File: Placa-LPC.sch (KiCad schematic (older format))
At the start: 17 parts, among them K1 CONN_3, P6 CONN_4X2, P7 CONN_8, P8 CONN_6, X1 12MHz

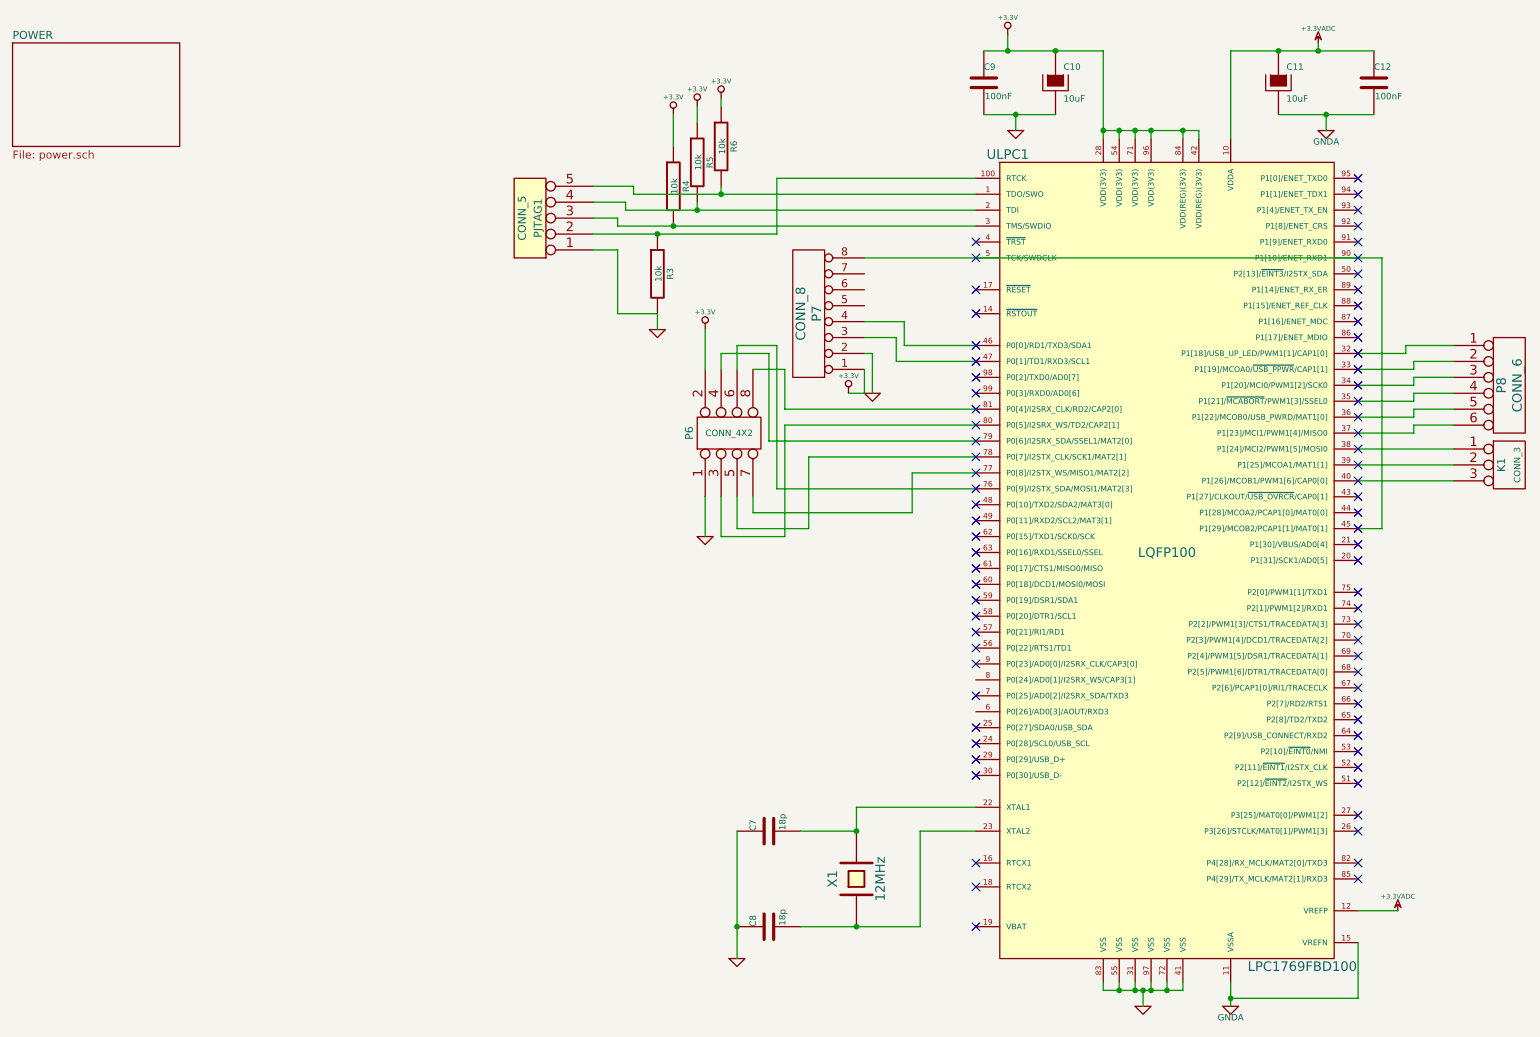
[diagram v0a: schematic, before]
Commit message: Actualizado desde mi pc
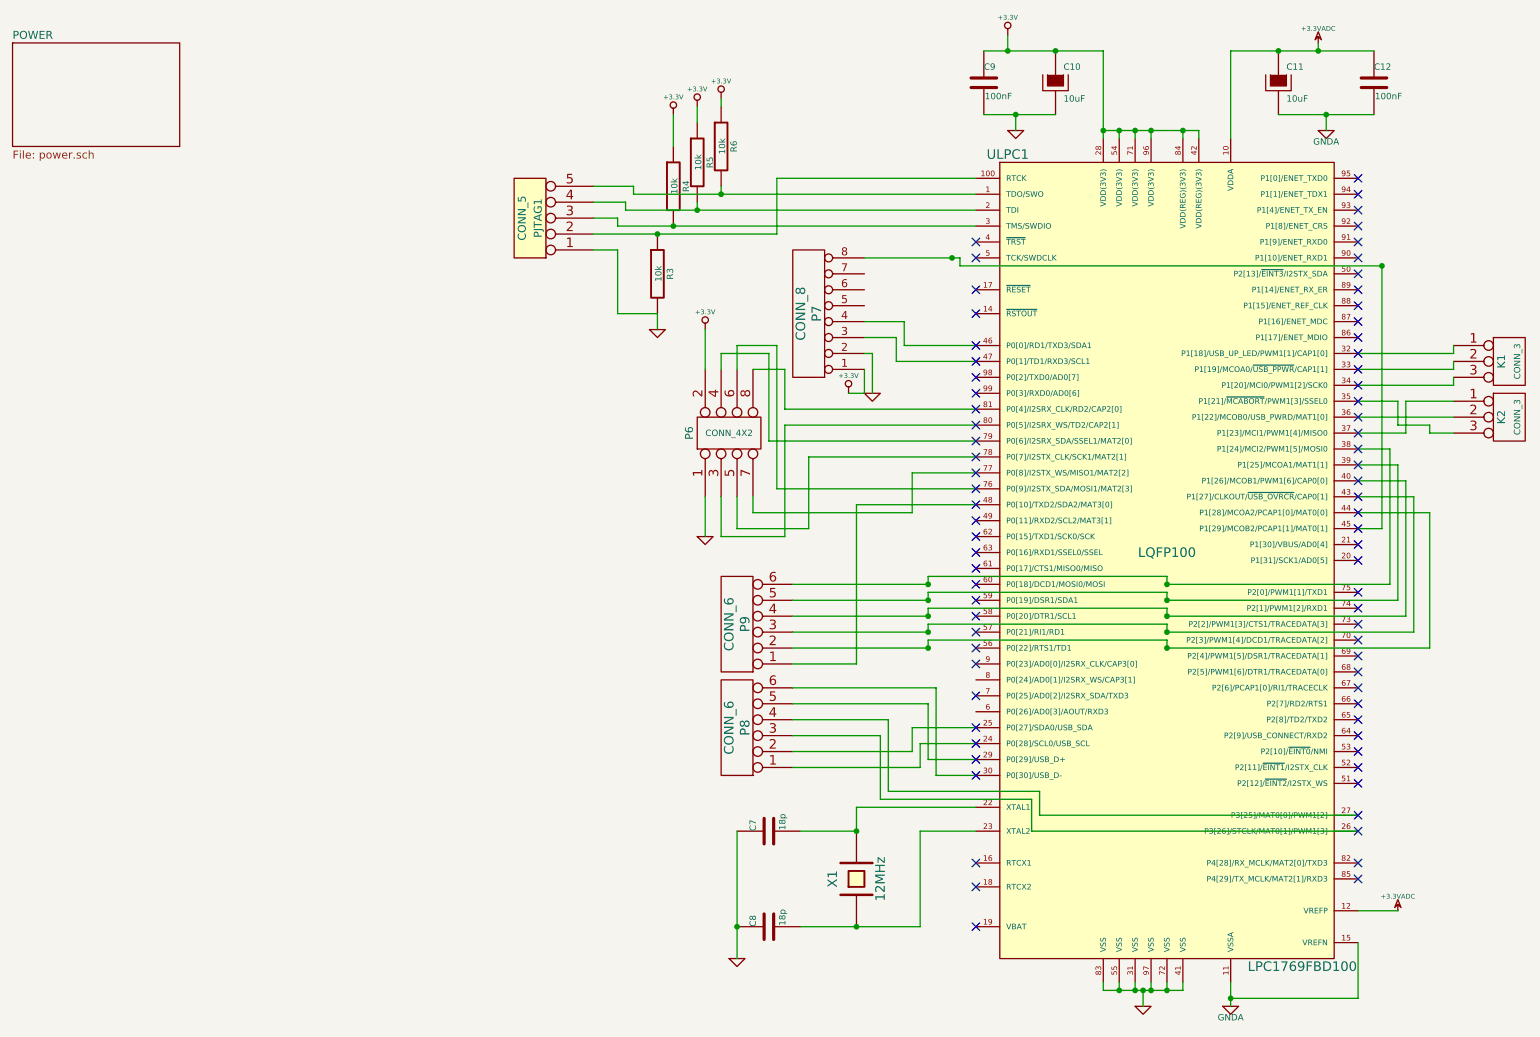
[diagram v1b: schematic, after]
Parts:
- added K2: CONN_3, symbol CONN_3
- added P9: CONN_6, symbol CONN_6
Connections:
- net at ULPC1.24 (P0[28]/SCL0/USB_SCL): now also P8.1
- net at ULPC1.25 (P0[27]/SDA0/USB_SDA): now also P8.2
- net at ULPC1.26 (P3[26]/STCLK/MAT0[1]/PWM1[3]): now also P8.3
- net at ULPC1.27 (P3[25]/MAT0[0]/PWM1[2]): now also P8.4
- net at ULPC1.29 (P0[29]/USB_D+): now also P8.5
- net at ULPC1.30 (P0[30]/USB_D-): now also P8.6
- net at ULPC1.32 (P1[18]/USB_UP_LED/PWM1[1]/CAP1[0]): now also K1.1 (P1); no longer P8.1
- net at ULPC1.33 (P1[19]/MCOA0/~USB_PPWR~/CAP1[1]): now also K1.2 (PM); no longer P8.2
- net at ULPC1.34 (P1[20]/MCI0/PWM1[2]/SCK0): now also K1.3 (P3); no longer P8.3
- net at ULPC1.35 (P1[21]/~MCABORT~/PWM1[3]/SSEL0): now also K2.3 (P3); no longer P8.4
- net at ULPC1.36 (P1[22]/MCOB0/USB_PWRD/MAT1[0]): now also K2.2 (PM); no longer P8.5
- net at ULPC1.37 (P1[23]/MCI1/PWM1[4]/MISO0): now also K2.1 (P1); no longer P8.6
- net at ULPC1.38 (P1[24]/MCI2/PWM1[5]/MOSI0): now also P9.6; no longer K1.1 (P1)
- net at ULPC1.39 (P1[25]/MCOA1/MAT1[1]): now also P9.5; no longer K1.2 (PM)
- net at ULPC1.40 (P1[26]/MCOB1/PWM1[6]/CAP0[0]): now also P9.4; no longer K1.3 (P3)
- net at ULPC1.43 (P1[27]/CLKOUT/~USB_OVRCR~/CAP0[1]): now also P9.3
- net at ULPC1.44 (P1[28]/MCOA2/PCAP1[0]/MAT0[0]): now also P9.2
- net at ULPC1.48 (P0[10]/TXD2/SDA2/MAT3[0]): now also P9.1
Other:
- moved on the sheet: K1, P8
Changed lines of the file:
@@
 Sheet 1 2
 Title ""
-Date "19 oct 2015"
+Date "20 oct 2015"
 Rev ""
 Comp ""
@@
 	6500 2700 6250 2700
 Wire Wire Line
-	6250 2300 9500 2300
+	6250 2300 6850 2300
 $Comp
 L CONN_6 P8
 U 1 1 56244F3D
-P 10300 3100
-F 0 "P8" V 10250 3100 60  0000 C CNN
-F 1 "CONN_6" V 10350 3100 60  0000 C CNN
-F 2 "" H 10300 3100 60  0000 C CNN
-F 3 "" H 10300 3100 60  0000 C CNN
-	1    10300 3100
-	1    0    0    -1
+P 5450 5250
+F 0 "P8" V 5400 5250 60  0000 C CNN
+F 1 "CONN_6" V 5500 5250 60  0000 C CNN
+F 2 "" H 5450 5250 60  0000 C CNN
+F 3 "" H 5450 5250 60  0000 C CNN
+	1    5450 5250
+	-1   0    0    1
 $EndComp
 $Comp
 L CONN_3 K1
 U 1 1 56244F4C
-P 10300 3600
-F 0 "K1" V 10250 3600 50  0000 C CNN
-F 1 "CONN_3" V 10350 3600 40  0000 C CNN
-F 2 "" H 10300 3600 60  0000 C CNN
-F 3 "" H 10300 3600 60  0000 C CNN
-	1    10300 3600
-	1    0    0    -1
-$EndComp
-Wire Wire Line
-	9350 2900 9650 2900
-Wire Wire Line
-	9650 2900 9650 2850
-Wire Wire Line
-	9650 2850 9950 2850
-Wire Wire Line
-	9950 2950 9700 2950
-Wire Wire Line
-	9700 2950 9700 3000
-Wire Wire Line
-	9700 3000 9350 3000
-Wire Wire Line
-	9350 3100 9700 3100
-Wire Wire Line
-	9700 3100 9700 3050
-Wire Wire Line
-	9700 3050 9950 3050
-Wire Wire Line
-	9350 3200 9700 3200
-Wire Wire Line
-	9700 3200 9700 3150
-Wire Wire Line
-	9700 3150 9950 3150
-Wire Wire Line
-	9350 3300 9700 3300
-Wire Wire Line
-	9700 3300 9700 3250
-Wire Wire Line
-	9700 3250 9950 3250
-Wire Wire Line
-	9350 3400 9700 3400
-Wire Wire Line
-	9700 3400 9700 3350
-Wire Wire Line
-	9700 3350 9950 3350
-Wire Wire Line
-	9350 3500 9950 3500
-Wire Wire Line
-	9350 3600 9950 3600
-Wire Wire Line
-	9350 3700 9950 3700
-Wire Wire Line
-	9500 2300 9500 4000
+P 10300 2950
+F 0 "K1" V 10250 2950 50  0000 C CNN
+F 1 "CONN_3" V 10350 2950 40  0000 C CNN
+F 2 "" H 10300 2950 60  0000 C CNN
+F 3 "" H 10300 2950 60  0000 C CNN
+	1    10300 2950
+	1    0    0    -1
+$EndComp
+Wire Wire Line
+	9500 2350 9500 4000
 Wire Wire Line
 	9500 4000 9350 4000
+$Comp
+L CONN_6 P9
+U 1 1 56269EC2
+P 5450 4600
+F 0 "P9" V 5400 4600 60  0000 C CNN
+F 1 "CONN_6" V 5500 4600 60  0000 C CNN
+F 2 "" H 5450 4600 60  0000 C CNN
+F 3 "" H 5450 4600 60  0000 C CNN
+	1    5450 4600
+	-1   0    0    1
+$EndComp
+$Comp
+L CONN_3 K2
+U 1 1 56269F4B
+P 10300 3300
+F 0 "K2" V 10250 3300 50  0000 C CNN
+F 1 "CONN_3" V 10350 3300 40  0000 C CNN
+F 2 "" H 10300 3300 60  0000 C CNN
+F 3 "" H 10300 3300 60  0000 C CNN
+	1    10300 3300
+	1    0    0    -1
+$EndComp
+Wire Wire Line
+	5800 4850 6200 4850
+Wire Wire Line
+	6200 4850 6200 3850
+Wire Wire Line
+	6200 3850 6950 3850
+Wire Wire Line
+	9350 3900 9800 3900
+Wire Wire Line
+	9800 3900 9800 4750
+Wire Wire Line
+	9800 4750 8150 4750
+Wire Wire Line
+	6650 4750 5800 4750
+Wire Wire Line
+	9350 3800 9700 3800
+Wire Wire Line
+	9700 3800 9700 4650
+Wire Wire Line
+	9700 4650 8150 4650
+Wire Wire Line
+	6650 4650 5800 4650
+Wire Wire Line
+	9350 3700 9650 3700
+Wire Wire Line
+	9650 3700 9650 4550
+Wire Wire Line
+	9650 4550 8150 4550
+Wire Wire Line
+	6650 4550 5800 4550
+Wire Wire Line
+	9350 3600 9600 3600
+Wire Wire Line
+	9600 3600 9600 4450
+Wire Wire Line
+	9600 4450 8150 4450
+Wire Wire Line
+	6650 4450 5800 4450
+Wire Wire Line
+	9350 3500 9550 3500
+Wire Wire Line
+	9550 3500 9550 4350
+Wire Wire Line
+	9550 4350 8150 4350
+Wire Wire Line
+	6650 4350 5800 4350
+Wire Wire Line
+	9350 3400 9650 3400
+Wire Wire Line
+	9650 3400 9650 3200
+Wire Wire Line
+	9650 3200 9950 3200
+Wire Wire Line
+	9350 3300 9950 3300
+Wire Wire Line
+	9350 3200 9600 3200
+Wire Wire Line
+	9600 3200 9600 3350
+Wire Wire Line
+	9600 3350 9800 3350
+Wire Wire Line
+	9800 3350 9800 3400
+Wire Wire Line
+	9800 3400 9950 3400
+Wire Wire Line
+	9350 3100 9950 3100
+Wire Wire Line
+	9950 3100 9950 3050
+Wire Wire Line
+	9950 2950 9950 3000
+Wire Wire Line
+	9950 3000 9350 3000
+Wire Wire Line
+	9350 2900 9950 2900
+Wire Wire Line
+	9950 2900 9950 2850
+Wire Wire Line
+	5800 5000 6700 5000
+Wire Wire Line
+	6700 5000 6700 5550
+Wire Wire Line
+	6700 5550 6950 5550
+Wire Wire Line
+	6950 5450 6650 5450
+Wire Wire Line
+	6650 5450 6650 5100
+Wire Wire Line
+	6650 5100 5800 5100
+Wire Wire Line
+	6950 5250 6550 5250
+Wire Wire Line
+	6550 5250 6550 5400
+Wire Wire Line
+	6550 5400 5800 5400
+Wire Wire Line
+	6950 5350 6600 5350
+Wire Wire Line
+	6600 5350 6600 5500
+Wire Wire Line
+	6600 5500 5800 5500
+Wire Wire Line
+	9350 5800 7350 5800
+Wire Wire Line
+	7350 5800 7350 5650
+Wire Wire Line
+	7350 5650 6400 5650
+Wire Wire Line
+	6400 5650 6400 5200
+Wire Wire Line
+	6400 5200 5800 5200
+Wire Wire Line
+	5800 5300 6350 5300
+Wire Wire Line
+	6350 5300 6350 5700
+Wire Wire Line
+	6350 5700 7300 5700
+Wire Wire Line
+	7300 5700 7300 5900
+Wire Wire Line
+	7300 5900 9350 5900
+Wire Wire Line
+	6650 4350 6650 4300
+Wire Wire Line
+	6650 4300 8150 4300
+Wire Wire Line
+	8150 4300 8150 4350
+Connection ~ 8150 4350
+Connection ~ 6650 4350
+Wire Wire Line
+	6650 4450 6650 4400
+Wire Wire Line
+	6650 4400 8150 4400
+Wire Wire Line
+	8150 4400 8150 4450
+Connection ~ 8150 4450
+Connection ~ 6650 4450
+Wire Wire Line
+	6650 4550 6650 4500
+Wire Wire Line
+	6650 4500 8150 4500
+Wire Wire Line
+	8150 4500 8150 4550
+Connection ~ 8150 4550
+Connection ~ 6650 4550
+Wire Wire Line
+	6650 4650 6650 4600
+Wire Wire Line
+	6650 4600 8150 4600
+Wire Wire Line
+	8150 4600 8150 4650
+Connection ~ 8150 4650
+Connection ~ 6650 4650
+Wire Wire Line
+	8150 4750 8150 4700
+Wire Wire Line
+	8150 4700 6650 4700
+Connection ~ 8150 4750
+Wire Wire Line
+	6650 4700 6650 4750
+Connection ~ 6650 4750
+Wire Wire Line
+	6850 2300 6850 2350
+Wire Wire Line
+	6850 2350 9500 2350
+Connection ~ 9500 2350
+Connection ~ 6800 2300
 $EndSCHEMATC
